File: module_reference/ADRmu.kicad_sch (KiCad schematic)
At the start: 7 parts, among them J101 Harting 09042326831, J102 10Vf, J103 10Vs, J104 7Vref, J105 Lo

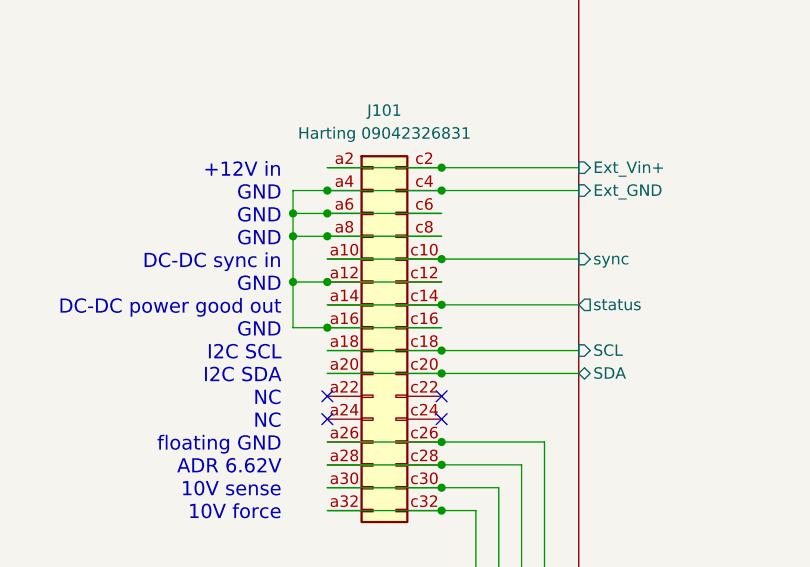
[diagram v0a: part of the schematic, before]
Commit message: asdf
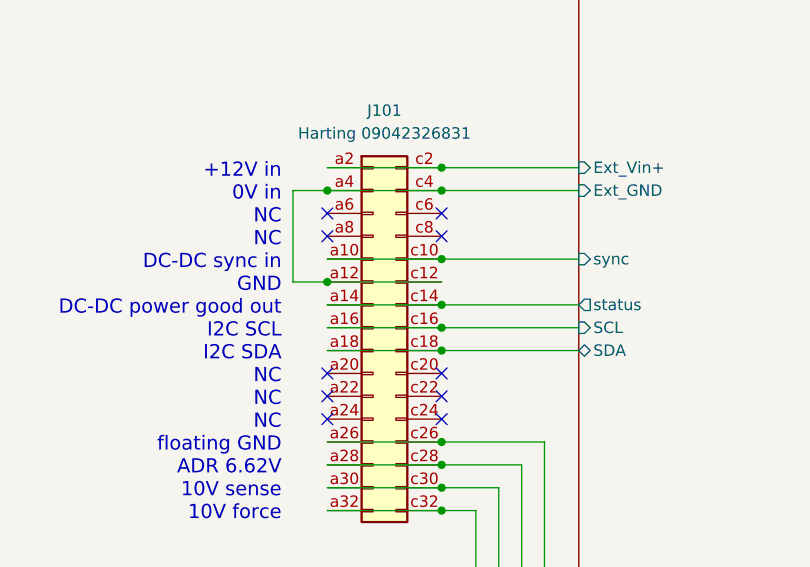
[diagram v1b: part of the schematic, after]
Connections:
- net DC-DC/Ext_GND: no longer J101.a16 (Pin_a16), J101.a6 (Pin_a6), J101.a8 (Pin_a8), J101.c16 (Pin_c16), J101.c6 (Pin_c6), J101.c8 (Pin_c8)
- net DC-DC/SCL: now also J101.a16 (Pin_a16), J101.c16 (Pin_c16); no longer J101.a18 (Pin_a18), J101.c18 (Pin_c18)
- net DC-DC/SDA: now also J101.a18 (Pin_a18), J101.c18 (Pin_c18); no longer J101.a20 (Pin_a20), J101.c20 (Pin_c20)
- no-connect marks 4 -> 10
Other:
- note added: "+12V in 0V in NC NC DC-DC sync in GND DC-DC power good out I2C SCL I2C SDA NC NC NC floating GND ADR 6.62V 10V sense 10V force"
- note removed: "+12V in GND GND GND DC-DC sync in GND DC-DC power good out GND I2C SCL I2C SDA NC NC floating GND ADR 6.62V 10V sense 10V force"
